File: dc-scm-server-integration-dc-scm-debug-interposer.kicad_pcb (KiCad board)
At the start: 6 copper layers, 90 x 69.9 mm, 164 parts, among them J1 Socket_DC-SCM-2.1_2x84_Rev-1-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, J10 PinHeader_2x5_P2.54mm_SMD, J11 PinHeader_2x5_P2.54mm_SMD, J12 PinHeader_2x5_P2.54mm_SMD, J13 PinHeader_2x5_P2.54mm_SMD, J15 Socket_SOP2-16_ACA-SPI-006-K0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, J16 Socket_SOP2-16_ACA-SPI-006-K0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, J17 PinHeader_2x5_P2.54mm_SMD, J2 PCB-Edge_DC-SCM-2.1_2x84_Rev-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, J3 PinHeader_2x5_P2.54mm_SMD, J4 PinHeader_2x5_P2.54mm_SMD, J5 PinHeader_2x5_P2.54mm_SMD, J6 PinHeader_2x5_P2.54mm_SMD, J7 PinHeader_2x5_P2.54mm_SMD, J9 PinHeader_2x5_P2.54mm_SMD, Q3 DMG1012T-7, U1 TLV76701_WSON

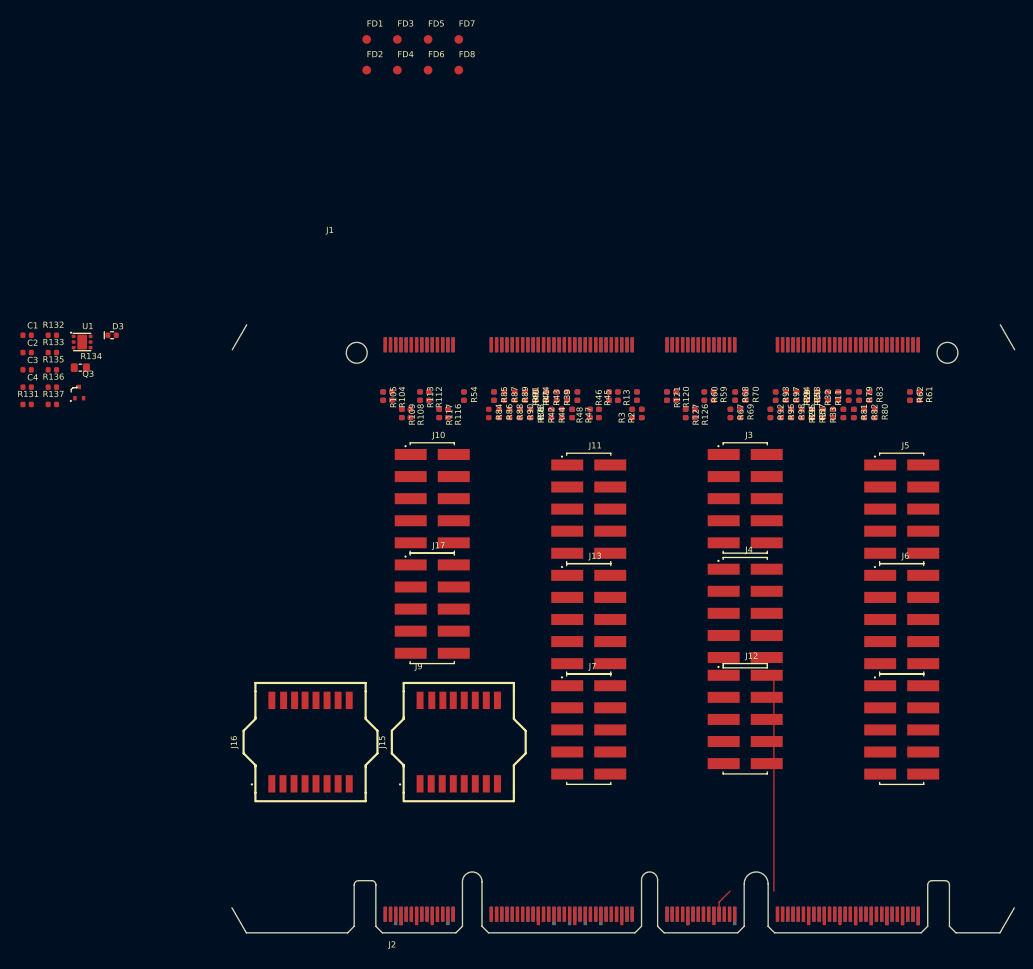
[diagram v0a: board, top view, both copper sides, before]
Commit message: [#100720] Finish placement
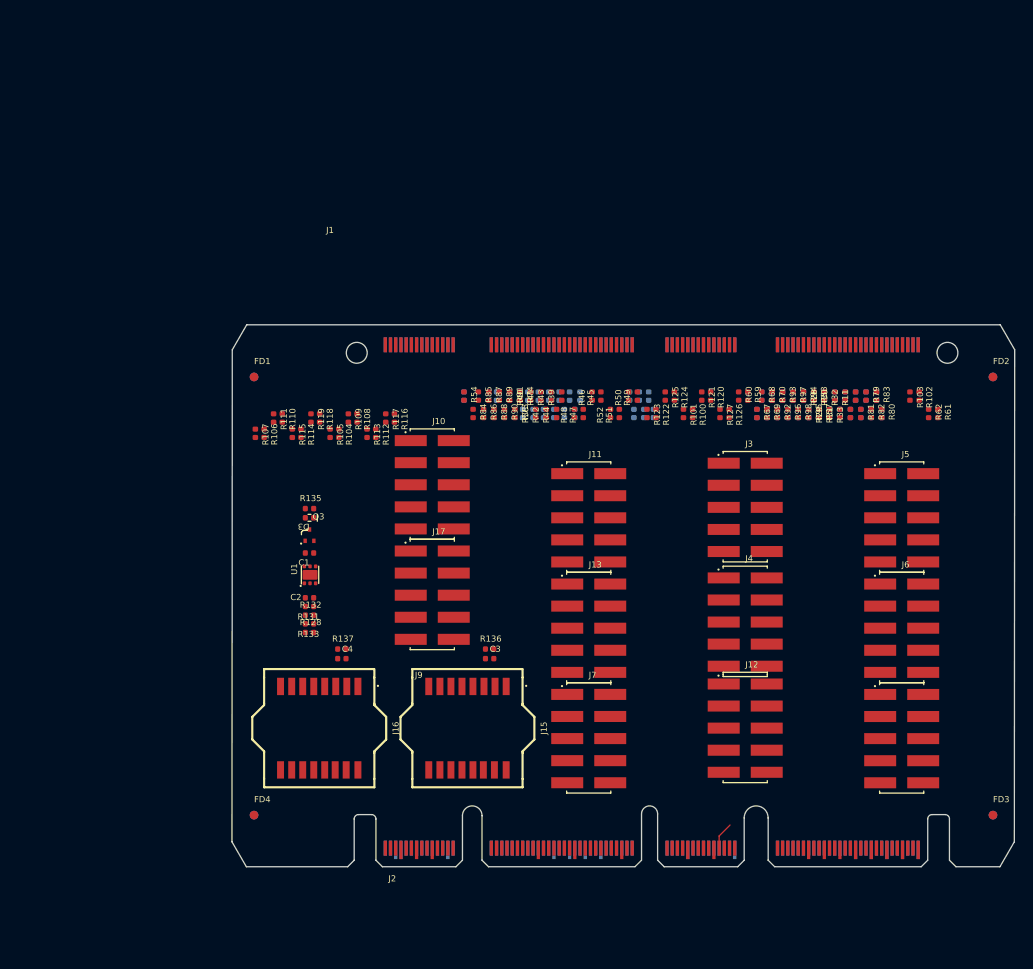
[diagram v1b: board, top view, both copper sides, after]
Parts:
- removed R134: R_0R_22.4A_0603, antmicro-footprints:R_0603_1608Metric
- added R128: R_0R_0402, antmicro-footprints:R_0402_1005Metric, F.Cu at (108.9, 105.4)
- FD5, FD6, FD7, FD8, R13, R2, R3: moved to B.Cu
- R100, R101, R102, R103, R106, R107, R110, R111, R114, R115, R118, R119, R122, R123, R124, R125, R49, R50, R51, R52: moved to F.Cu
- moved FD3 112.5 mm to (187.5, 126.4)
- moved FD7 108.3 mm to (187.5, 126.4), turned to 180 degrees
- moved FD8 88.9 mm to (102.5, 126.4), turned to 180 degrees
- moved FD4 87.3 mm to (102.5, 126.4)
- moved FD2 80.2 mm to (187.5, 76.0)
- moved FD6 73.9 mm to (187.5, 76.0), turned to 180 degrees
- moved C3 62.7 mm to (129.6, 108.4)
- moved R136 58.6 mm to (129.6, 107.3)
- moved C4 47.8 mm to (112.6, 108.4)
- moved R132 43.7 mm to (108.9, 103.4)
- moved FD5 43.7 mm to (102.5, 76.0), turned to 180 degrees
- moved R137 43.6 mm to (112.6, 107.3)
- moved C2 43.0 mm to (108.9, 101.4), turned to 180 degrees
- moved R133 43.0 mm to (108.9, 104.4), turned to 180 degrees
- moved C1 41.0 mm to (108.9, 96.2), turned to 180 degrees
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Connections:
- J7 pad 10: GND -> /DC-SCI edge connector/DC_SCM_I2C_I3C19.SCL
- J7 pad 3: /DC-SCI edge connector/DC_SCM_I2C_I3C18.SCL -> GND
- J7 pad 6: GND -> /DC-SCI edge connector/DC_SCM_I2C_I3C18.SCL
- J7 pad 7: /DC-SCI edge connector/DC_SCM_I2C_I3C19.SCL -> GND
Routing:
- net /DC-SCI edge connector/DC_SCM_I2C_I3C14.SCL: track 27.9 -> 3.18 mm
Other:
- board size 90 x 69.9 mm -> 90 x 62.3 mm
